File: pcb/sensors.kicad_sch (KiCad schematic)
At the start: 20 parts, among them J2 Conn_01x04_Pin, Q1 BSS138, U3 BME280, U4 SGP30-2.5K

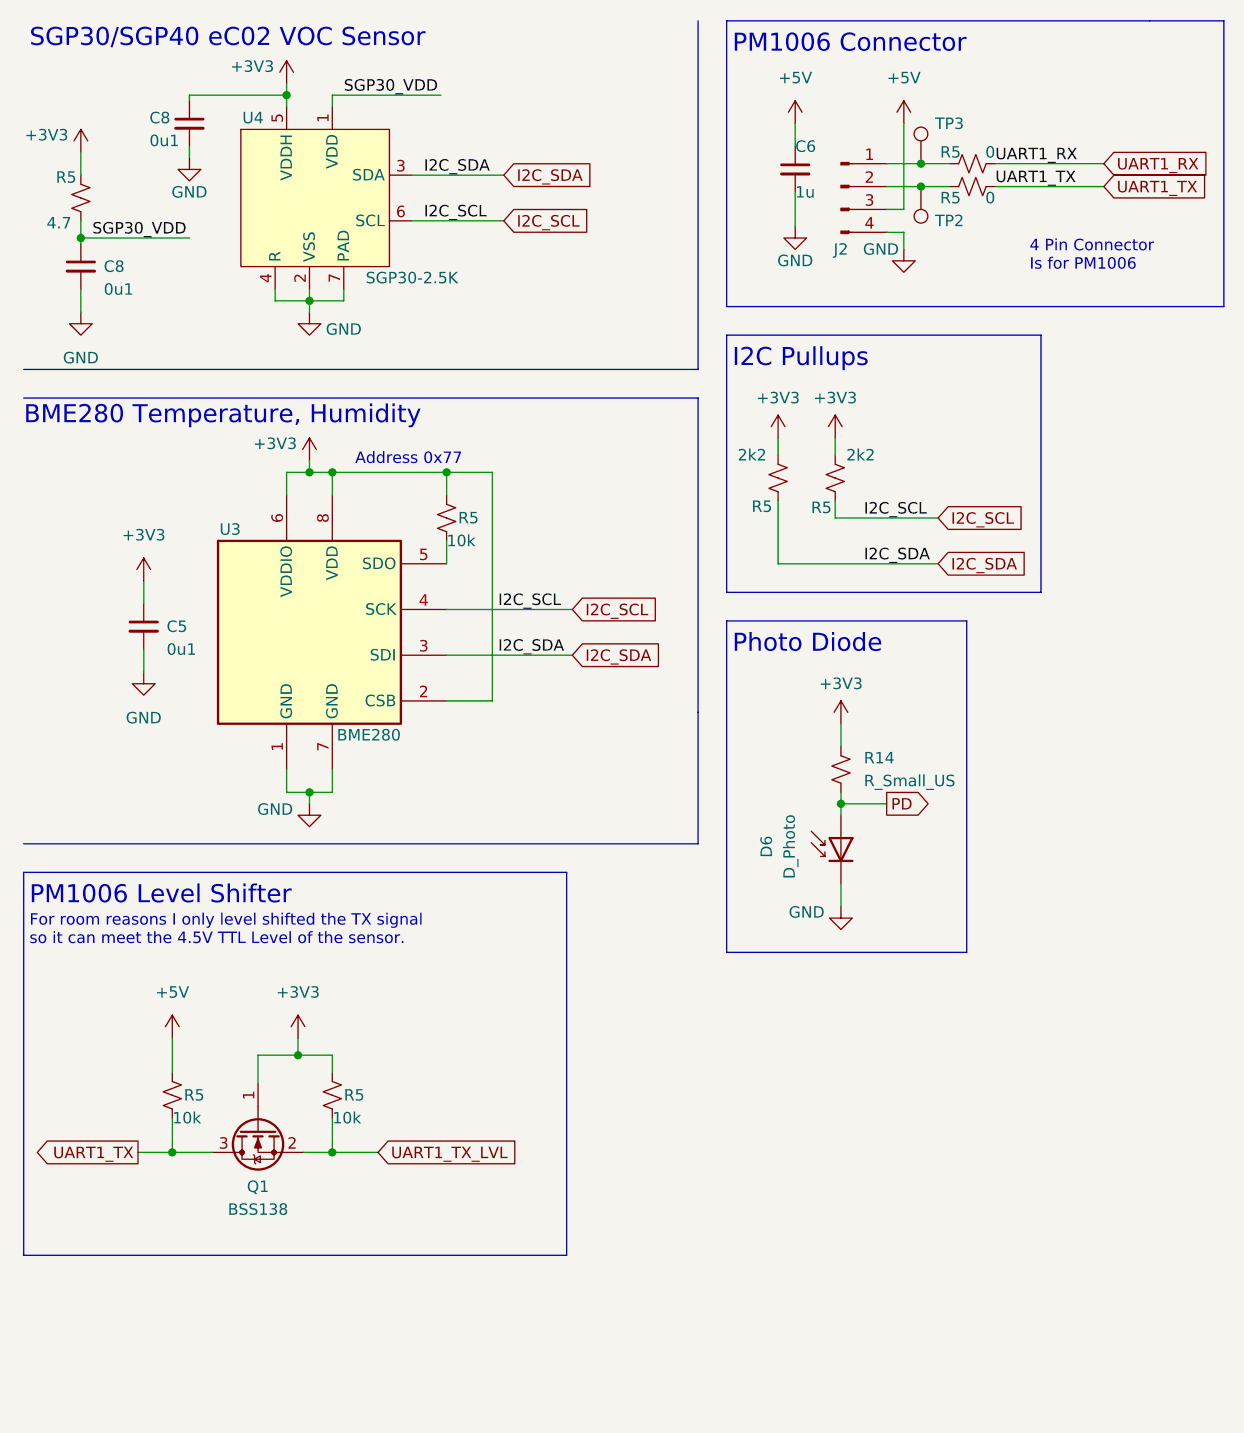
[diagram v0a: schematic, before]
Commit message: README
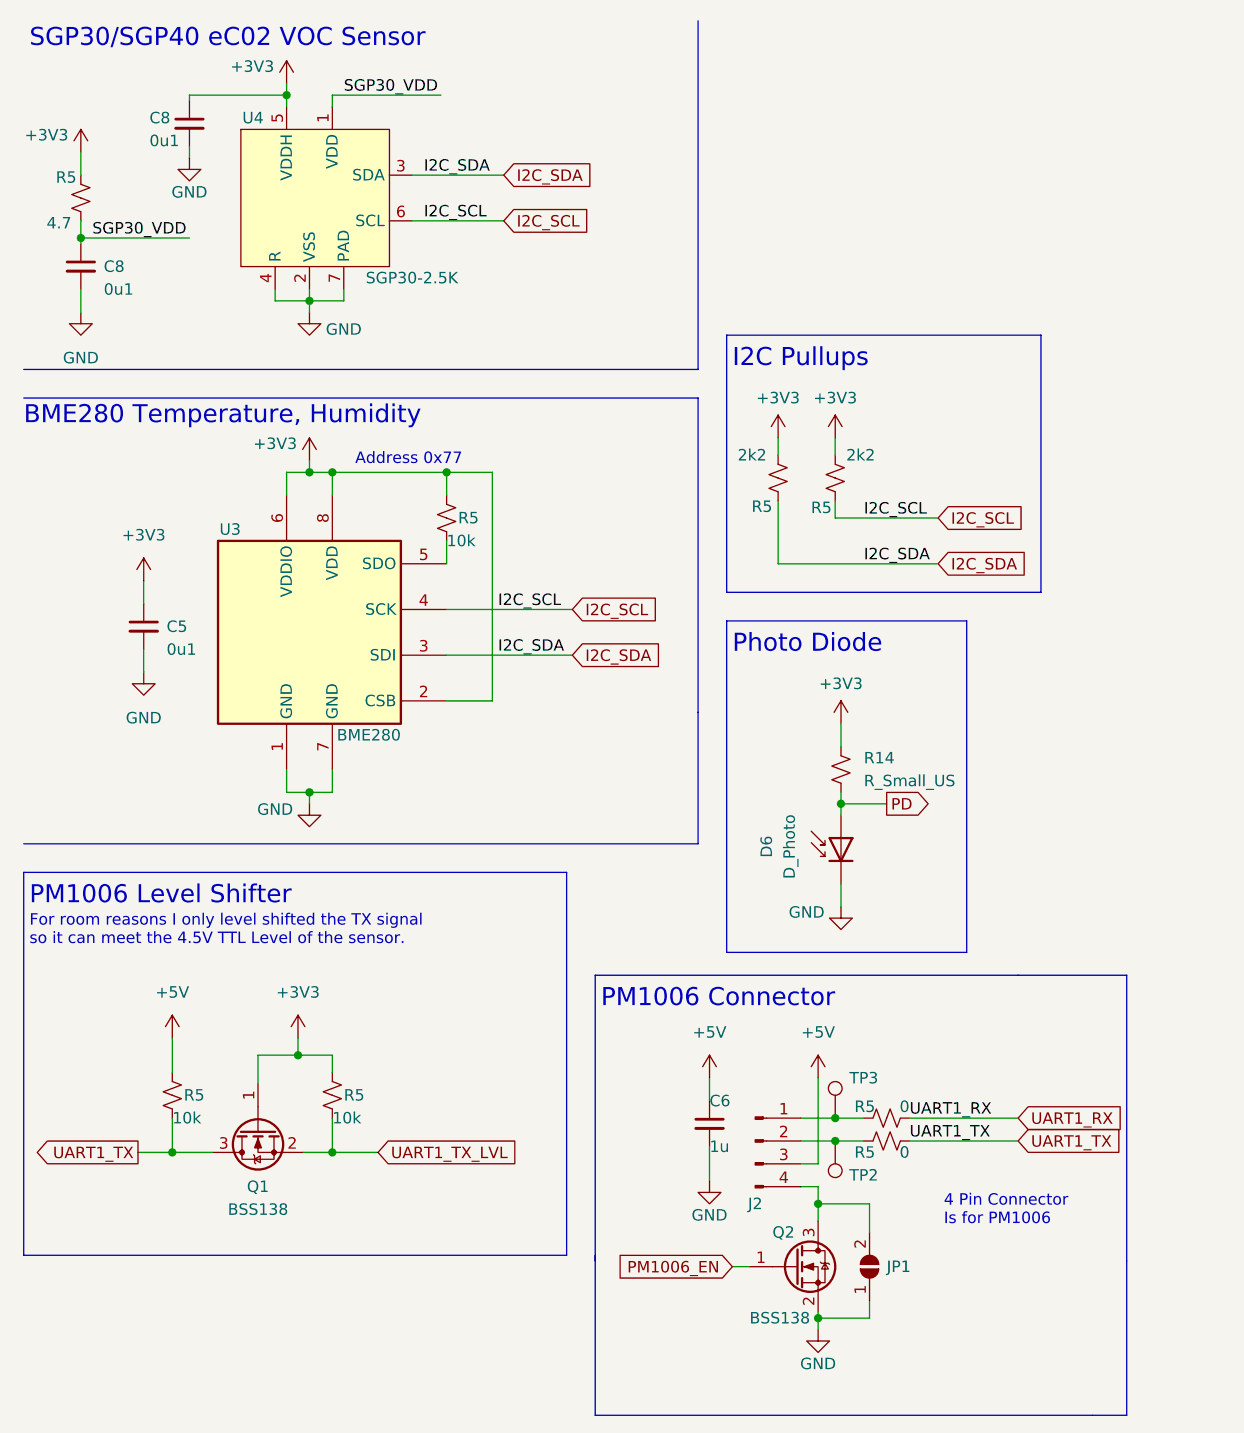
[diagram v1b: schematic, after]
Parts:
- added JP1: SolderJumper_2_Open, Jumper:SolderJumper-2_P1.3mm_Open_RoundedPad1.0x1.5mm, symbol Jumper:SolderJumper_2_Open
- added Q2: BSS138, Package_TO_SOT_SMD:SOT-23, symbol Transistor_FET:BSS138
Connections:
- net GND: now also JP1.1 (A), Q2.2 (S); no longer J2.4 (Pin_4)
- new net: J2.4 (Pin_4), JP1.2 (B), Q2.3 (D)
- new net PM1006_EN: Q2.1 (G)
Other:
- moved on the sheet: C6, J2, R5, TP2, TP3
